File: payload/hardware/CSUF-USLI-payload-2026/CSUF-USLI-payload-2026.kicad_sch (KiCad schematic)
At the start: 3 parts, among them U1 DEV-16771, U2 GPS6MV2

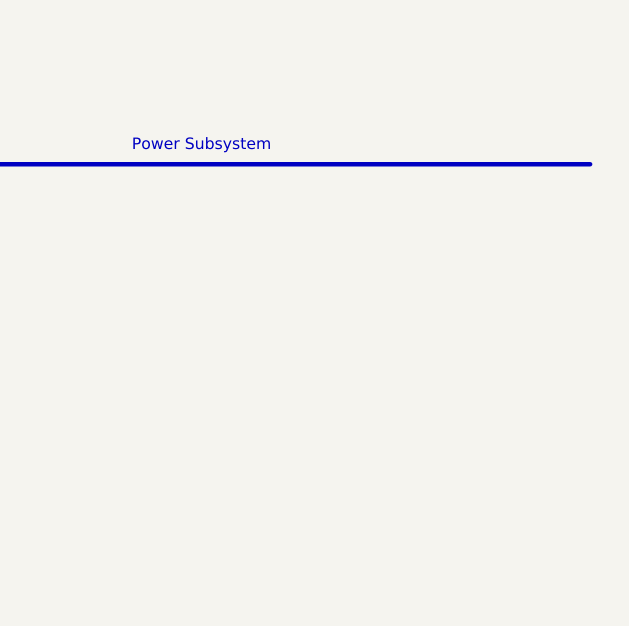
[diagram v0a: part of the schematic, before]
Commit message: Motor Diagram Concept
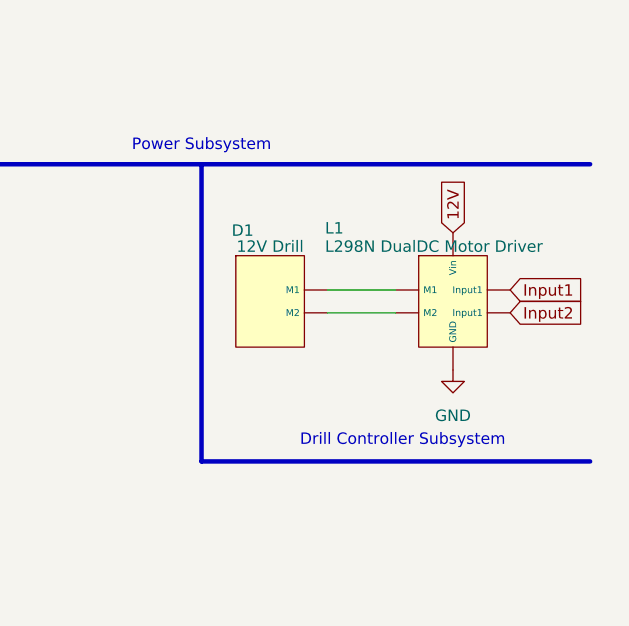
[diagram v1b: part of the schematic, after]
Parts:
- added D1: 12V Drill, symbol L298N Concept:12V_Drill
- added L1: L298N DualDC Motor Driver, symbol L298N Concept:L298N
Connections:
- net GND: now also L1. (Input1)
- new net: D1. (M2), L1. (Input1) (x2)
- new net 12V: L1. (Input1)
- new net Input1: L1. (Input1)
- new net Input2: L1. (Input1)
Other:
- note added: "Drill Controller Subsystem"
